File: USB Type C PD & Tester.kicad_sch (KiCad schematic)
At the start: 60 parts, among them J1 USB_B_Micro, J2 USB_C_Receptacle_USB2.0_14P, J3 USB_C_Receptacle_USB2.0_14P, Q1 BSD840N, Q2 BSD840N, Q3 BSD840N, Q4 BSD840N, SW1 SW_Push, U1 MIC5504-1.2YM5, U2 STM32F072CBTx, U3 INA237, U4 INA237, U5 AD8606ARM, U6 AD8606ARM

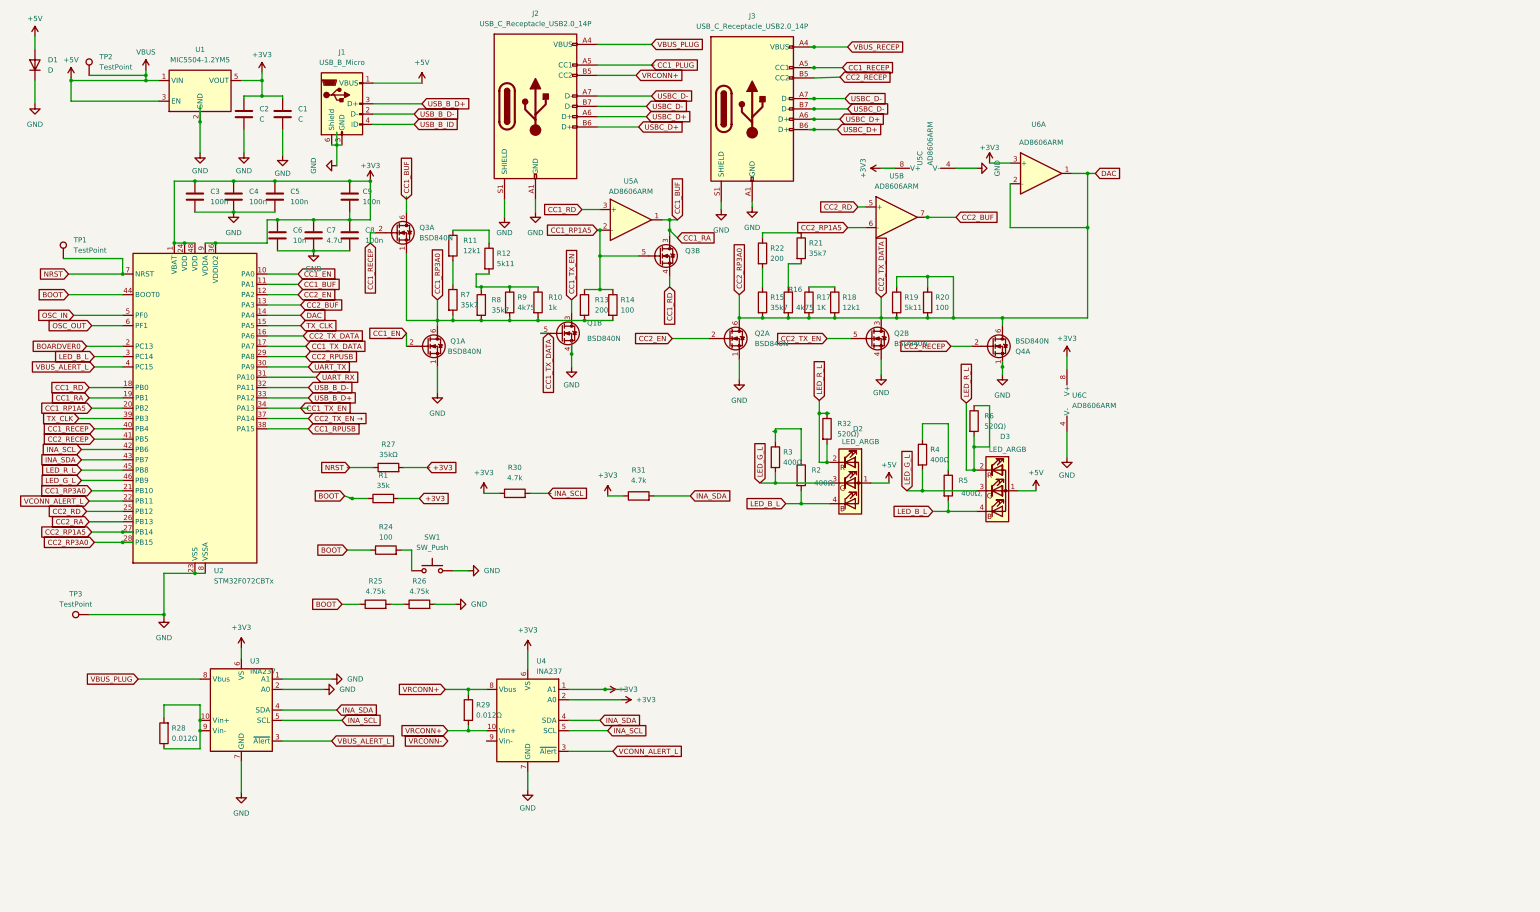
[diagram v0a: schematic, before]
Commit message: Add files via upload
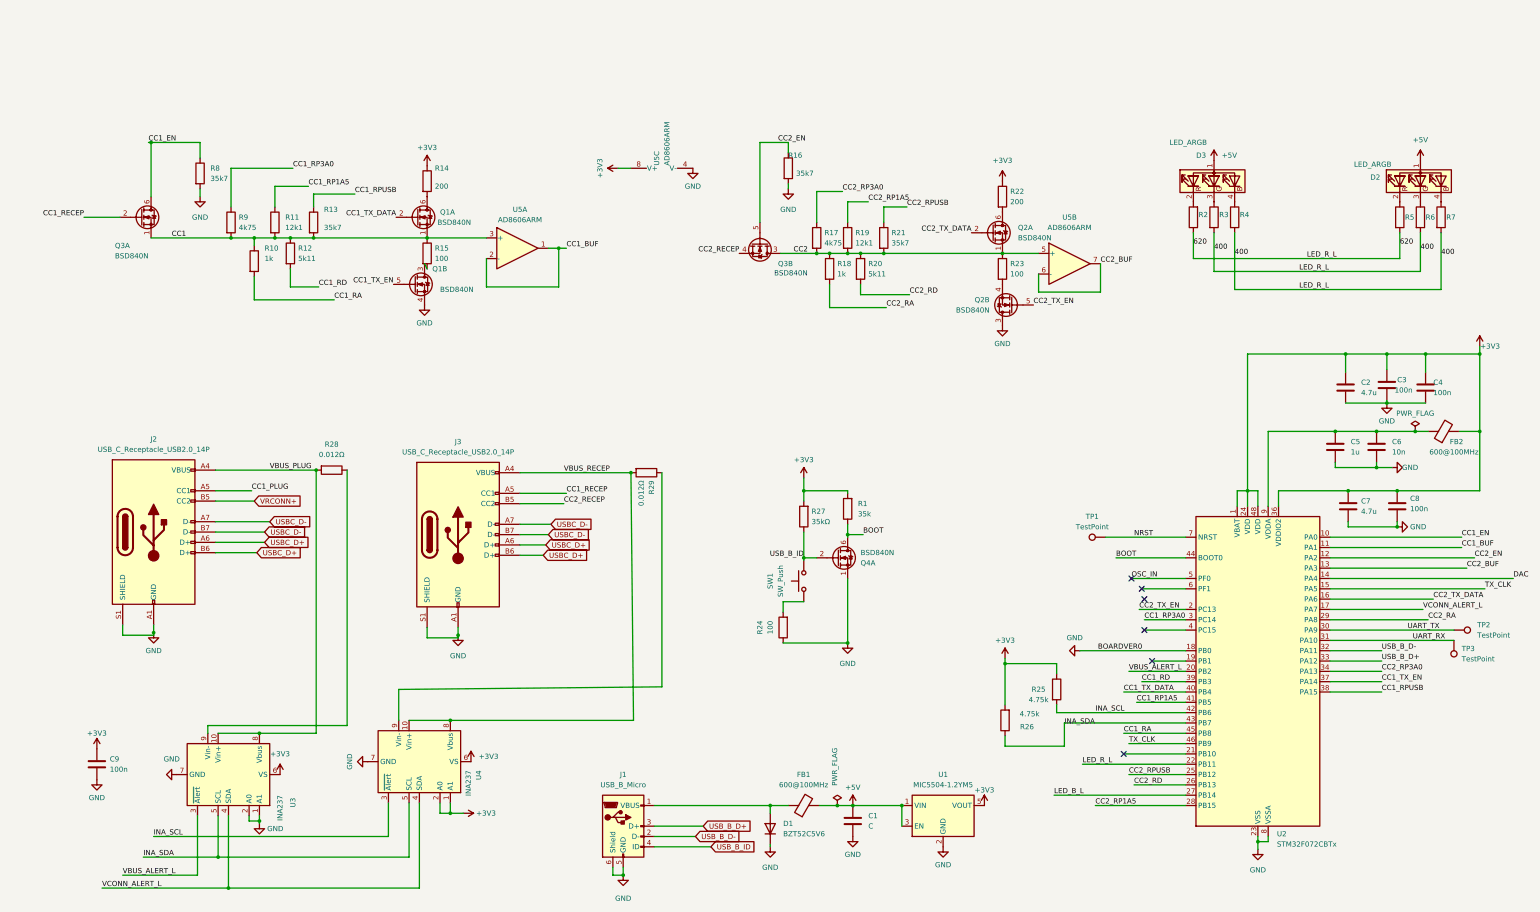
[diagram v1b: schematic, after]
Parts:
- removed R30, R31: 4.7k, Resistor_SMD:R_0402_1005Metric, symbol Device:R
- removed R7: 35k7, Resistor_SMD:R_0402_1005Metric, symbol Device:R
- removed U6: AD8606ARM, Package_SO:MSOP-8_3x3mm_P0.65mm, symbol Amplifier_Operational:AD8606ARM
- added FB1, FB2: 600@100MHz, symbol Device:FerriteBead
- added R23: 100, Resistor_SMD:R_0402_1005Metric, symbol Device:R
- C2: value C -> 4.7u
- C5: value 100n -> 1u
- D1: value D -> BZT52C5V6
- R13: value 200 -> 35k7
- R14: value 100 -> 200
- R15: value 35k7 -> 100
- R16: value 4k75 -> 35k7
- R17: value 1K -> 4k75
- R18: value 12k1 -> 1k
- R19: value 5k11 -> 12k1
- R2: renamed from R4; value 400Ω -> ~
- R20: value 100 -> 5k11
- R3: renamed from R6; value 520Ω) -> ~
- R4: renamed from R5; value 400Ω, -> ~
- R5: renamed from R3; value 400Ω -> ~
- R6: renamed from R32; value 520Ω) -> ~
- R7: renamed from R2; value 400Ω, -> ~
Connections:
- net BOARDVER0 is gone; now on net CC2_TX_EN: U2.2 (PC13)
- net CC2_TX_EN → is gone; now on net CC1_TX_EN: U2.37 (PA14)
- net +3V3: now also R14.1, R22.1, R25.1, R26.2, FB2.2; no longer C1.1, C5.1, C6.1, C9.2, U2.9 (VDDA)
- net +5V: now also C1.1, FB1.2; no longer D1.2 (A), J1.1 (VBUS), TP2.1
- net BOOT: now also Q4.6 (D); no longer R24.1, R25.1
- net CC1_BUF: now also U5.2 (-); no longer Q3.3 (D), Q3.6 (D), U2.19 (PB1)
- net CC1_EN: now also Q3.6 (D), R8.1; no longer Q1.2 (G)
- net CC1_RD: now also R12.2, U2.39 (PB3); no longer Q3.4 (S), U2.18 (PB0), U5.3 (+)
- net CC1_RECEP: no longer U2.40 (PB4)
- net CC1_RP1A5: now also R11.1, U2.41 (PB5); no longer Q3.5 (G), R13.1, R14.1, U2.20 (PB2), U5.2 (-)
- net CC1_RP3A0: now also R9.1, U2.3 (PC14); no longer Q1.6 (D), Q3.1 (S), R10.2, R13.2, R14.2, R8.2, R9.2, U2.21 (PB10)
- net CC1_RPUSB: now also R13.1
- net CC1_TX_DATA: now also Q1.2 (G), U2.40 (PB4); no longer Q1.5 (G), U2.17 (PA7)
- net CC1_TX_EN: now also Q1.5 (G); no longer Q1.3 (D), U2.34 (PA13)
- net CC2_BUF: now also U5.6 (-)
- net CC2_EN: now also Q3.5 (G), R16.1; no longer Q2.2 (G)
- net CC2_RA: now also R18.2, U2.29 (PA8); no longer U2.26 (PB13)
- net CC2_RD: now also R20.2, U2.26 (PB13); no longer U2.25 (PB12), U5.5 (+)
- net CC2_RECEP: now also Q3.4 (S); no longer Q4.2 (G), U2.41 (PB5)
- net CC2_RP1A5: now also R19.1, U2.28 (PB15); no longer U2.27 (PB14), U5.6 (-)
- net CC2_RP3A0: now also R17.1, U2.34 (PA13); no longer Q2.3 (D), Q2.6 (D), Q4.6 (D), R15.2, R16.2, R17.2, R18.2, R19.1, R19.2, R20.1, R20.2, U2.14 (PA4), U2.16 (PA6), U2.28 (PB15)
- net CC2_RPUSB: now also R21.1, U2.25 (PB12); no longer U2.29 (PA8)
- net GND: now also C9.2, Q2.3 (D), R16.2, R24.1, R8.2, U2.18 (PB0); no longer Q1.1 (S), Q2.1 (S), Q2.4 (S), R26.2, SW1.2, TP3.1
- net INA_SCL: now also R25.2, U4.3 (~{Alert}); no longer U3.5 (SCL), U4.5 (SCL)
- net INA_SDA: now also R26.1, U3.5 (SCL), U4.5 (SCL); no longer U3.4 (SDA), U4.4 (SDA)
- net LED_B_L: now also U2.27 (PB14); no longer D2.4 (BK), D3.4 (BK), R4.2, R7.2, U2.3 (PC14)
- net NRST: no longer R27.1
- net TX_CLK: now also U2.46 (PB9); no longer U2.39 (PB3)
- net UART_RX: now also TP3.1
- net UART_TX: now also TP2.1
- net USB_B_ID: now also Q4.2 (G), R27.1, SW1.2
- net VBUS_ALERT_L: now also U2.20 (PB2); no longer U2.4 (PC15)
- net VBUS_PLUG: now also R28.2, U3.10 (Vin+)
- net VBUS_RECEP: now also R29.2, U4.10 (Vin+), U4.8 (Vbus)
- net VCONN_ALERT_L: now also U2.17 (PA7), U3.4 (SDA), U4.4 (SDA); no longer U2.22 (PB11), U4.3 (~{Alert})
- net VRCONN+: no longer R29.1, R29.2, U4.10 (Vin+), U4.8 (Vbus)
- net at R5.1: now also D2.2 (RK); no longer R7.1
- net CC2: now reaches R18.1
- net CC2: now also Q2.1 (S), Q3.3 (D), R17.2, R19.2, R20.1, R21.2, U5.5 (+), R23.1; no longer R17.1
- net at U4.9 (Vin-): now also R29.1
- net CC1: now reaches R12.1
- net CC1: now also Q1.1 (S), Q3.1 (S), R10.1, R11.2, R13.2, R15.1, R9.2, U5.3 (+); no longer R11.1
- net at R4.1: now also D3.4 (BK); no longer R2.1
- net at R28.1, U3.9 (Vin-): no longer R28.2, U3.10 (Vin+)
- net at R22.2: now also Q2.6 (D); no longer R15.1
- removed net LED_G_L: D2.3 (GK), D3.3 (GK), R2.2, R5.2, U2.46 (PB9)
- removed net LED_R_L: D2.2 (RK), D3.2 (RK), R3.1, R3.2, R6.1, R6.2, U2.45 (PB8)
- net OSC_OUT: no longer names the net of U2.6 (PF1)
- new net: Q2.4 (S), R23.2
- new net: D1.2 (A), FB1.1, J1.1 (VBUS)
- new net: D2.3 (GK), R6.1
- new net: Q1.6 (D), R14.2
- new net: D3.2 (RK), R2.2
- new net: D3.3 (GK), R3.1
- new net: C5.1, C6.1, FB2.1, U2.9 (VDDA)
- new net: Q1.3 (D), R15.2
- new net: D2.4 (BK), R7.1
- new net 400: R2.1, R3.2, R4.2, R5.2, R6.2, R7.2, U2.22 (PB11)
- new net CC1_RA: R10.2, U2.45 (PB8)
- new net CC2_TX_DATA: Q2.2 (G), U2.16 (PA6)
- new net DAC: U2.14 (PA4)
- no-connect marks 0 -> 6
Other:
- note added: "BSD840N"
- moved on the sheet: C1, C2, C3, C4, C5, C6, C7, C8, C9, D1, D2, D3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
